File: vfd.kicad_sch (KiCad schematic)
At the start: 6 parts, among them J2 Conn_02x10_Counter_Clockwise, J3 Conn_02x10_Counter_Clockwise, U1 IV-18, U9 DRV8837

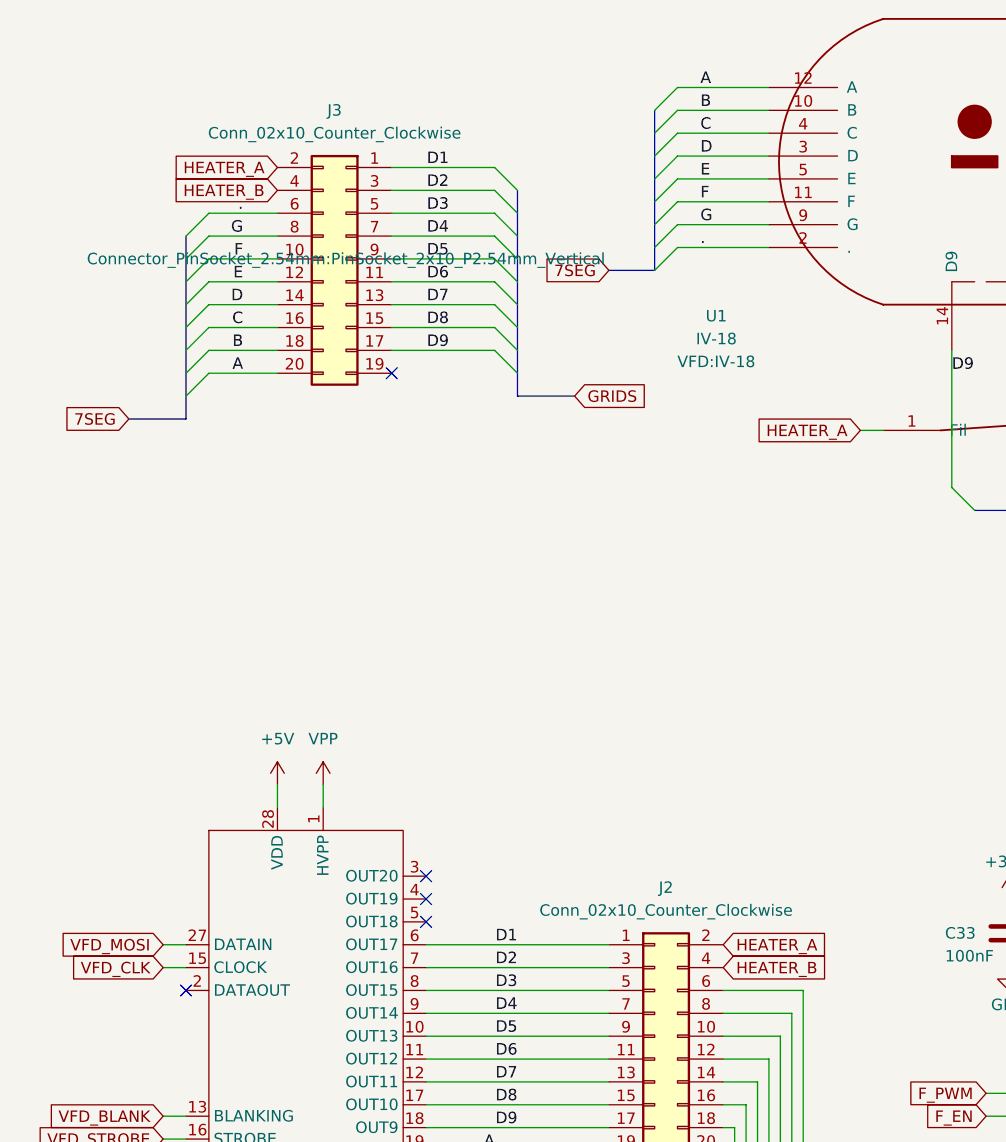
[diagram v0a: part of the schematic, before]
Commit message: Route some
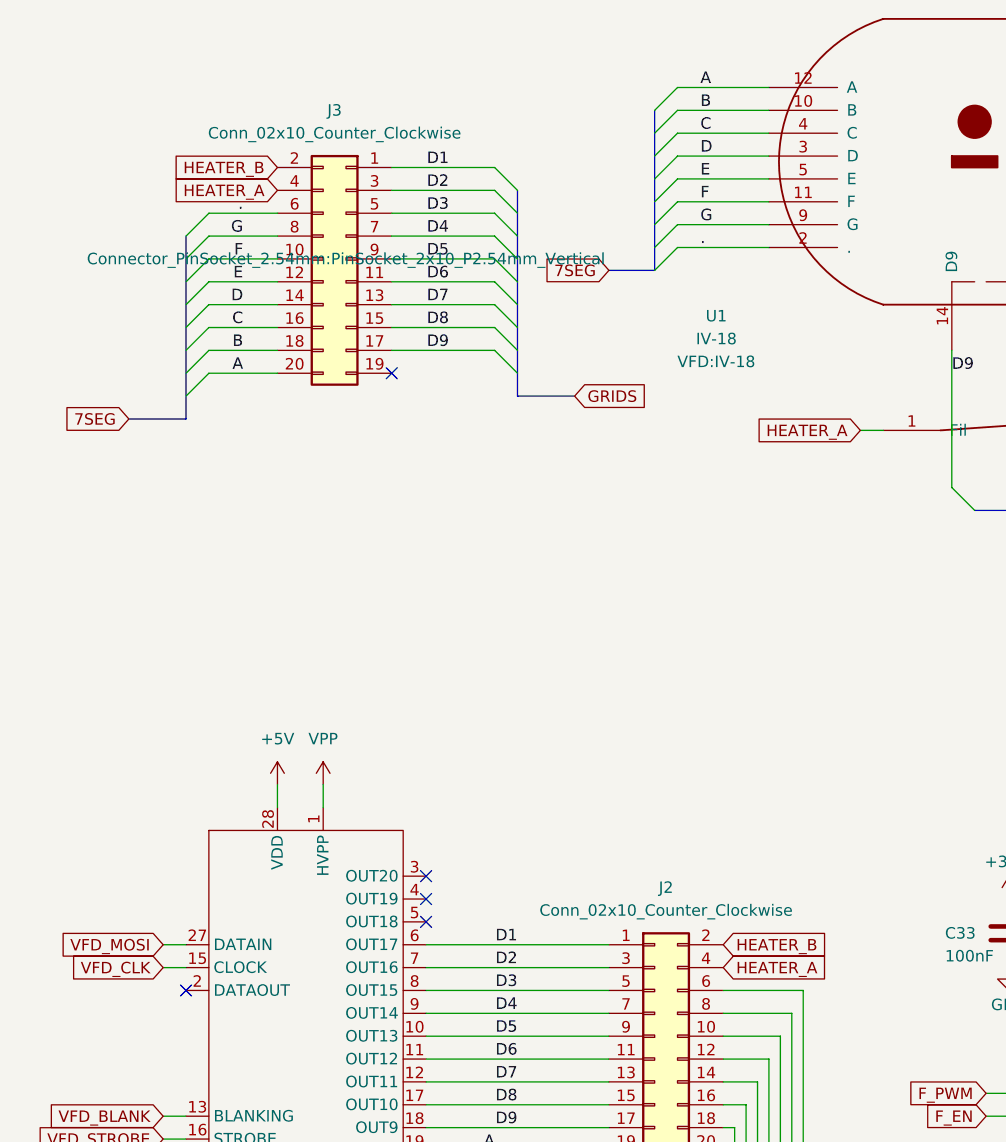
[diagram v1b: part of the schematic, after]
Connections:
- net HEATER_A: now also J2.4 (Pin_4), J3.4 (Pin_4); no longer J2.2 (Pin_2), J3.2 (Pin_2)
- net HEATER_B: now also J2.2 (Pin_2), J3.2 (Pin_2); no longer J2.4 (Pin_4), J3.4 (Pin_4)
